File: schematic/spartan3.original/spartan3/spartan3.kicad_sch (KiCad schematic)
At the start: 245 parts, among them U1_clk_select_0 SPFT_Sliding_Switch-dynacore, U2 XC3S250E-4TQG144C

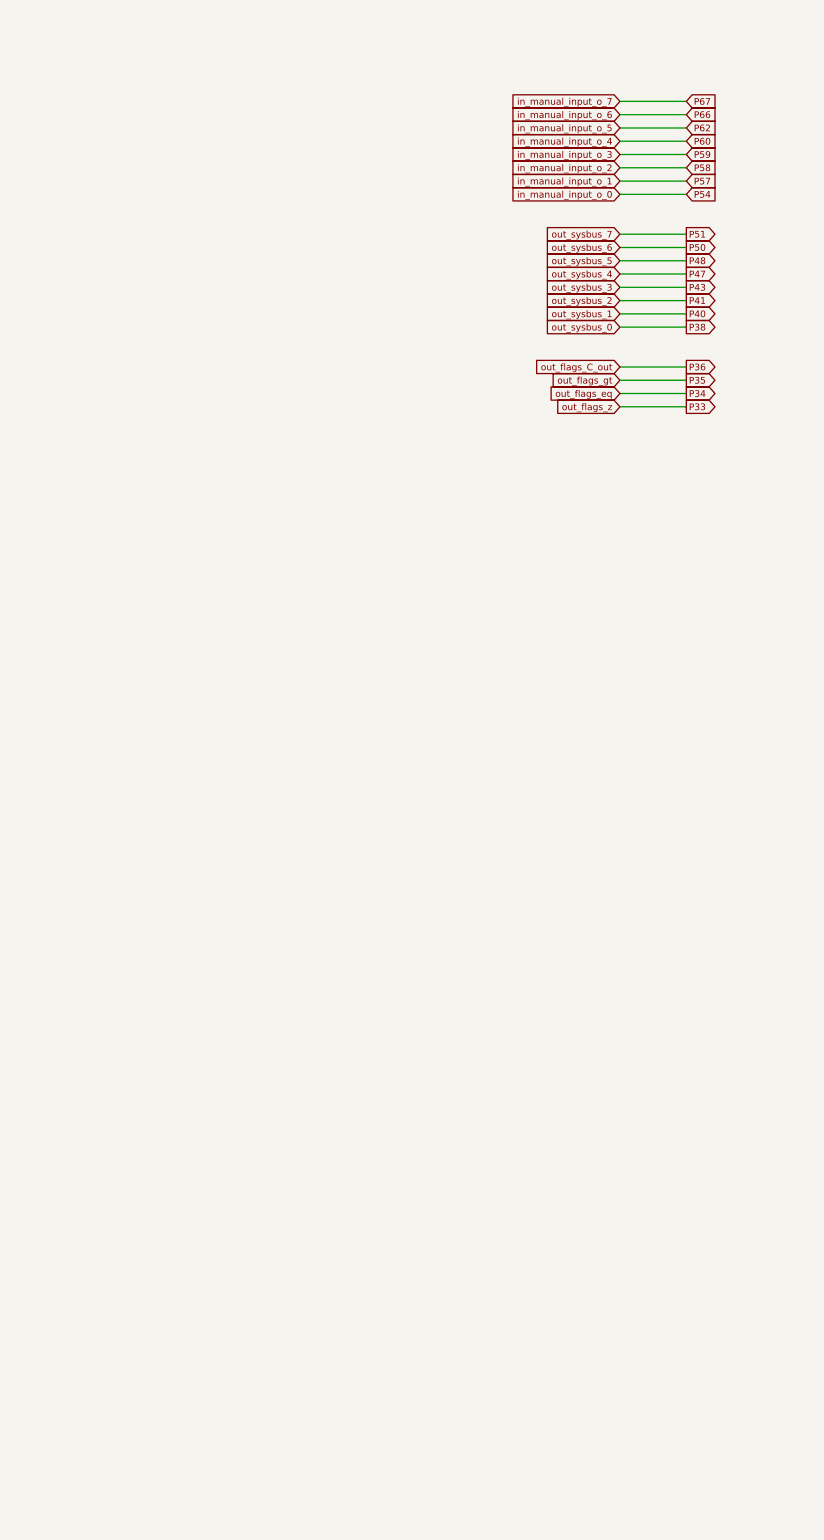
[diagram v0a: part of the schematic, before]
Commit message: Schematics :: updated. PCB layout :: updated
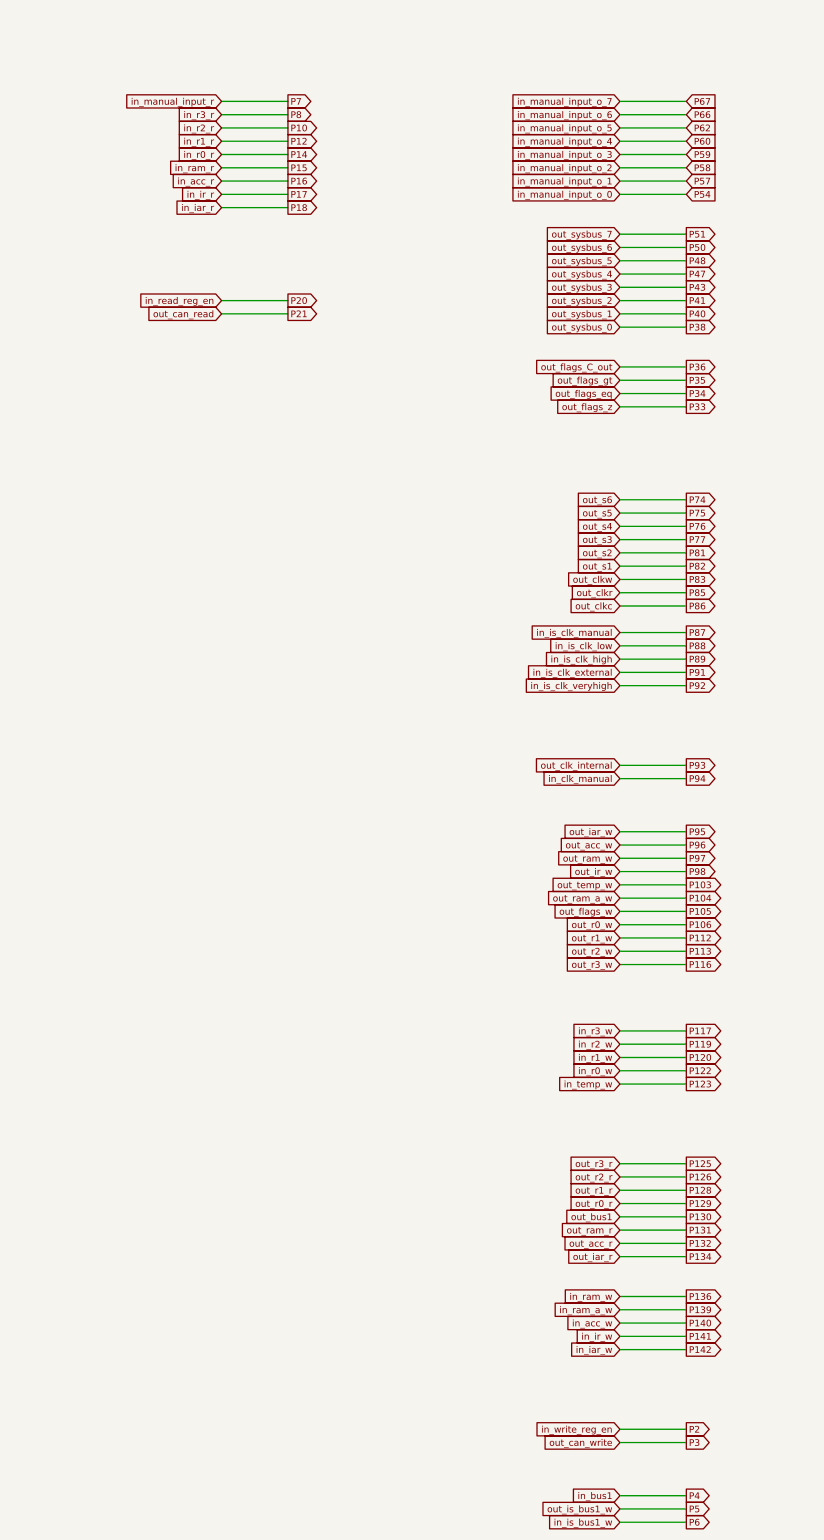
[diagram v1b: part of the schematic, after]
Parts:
- J_pwr_0: footprint Connector_USB:USB_A_Molex_67643_Horizontal -> Connector_USB:USB_A_Molex_105057_Vertical
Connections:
- net in_acc_r is gone; now on net P16: D_in_acc_r_0.1 (K), R_in_acc_r_0.1, SW_read_register_0.7
- net in_acc_w is gone; now on net P140: D_in_acc_w_0.1 (K), R_in_acc_w_0.1, SW_in_acc_w_0.5 (B)
- net in_bus1 is gone; now on net P4: D_in_bus1_one_0.1 (K), D_in_bus1_ps_0.2 (A), R_in_bus1_0.1, SW_in_bus1_0.2 (B)
- net in_clk_manual is gone; now on net P94: D_in_clk_manual_0.1 (K), R_in_clk_manual_0.1, SW_in_clk_manual_0.1
- net in_iar_r is gone; now on net P18: D_in_iar_r_0.1 (K), R_in_iar_r_0.1, SW_read_register_0.5
- net in_iar_w is gone; now on net P142: D_in_iar_w_0.1 (K), R_in_iar_w_0.1, SW_in_iar_w_0.5 (B)
- net in_ir_r is gone; now on net P17: D_in_ir_r_0.1 (K), R_in_ir_r_0.1, SW_read_register_0.6
- net in_ir_w is gone; now on net P141: D_in_ir_w_0.1 (K), R_in_ir_w_0.1, SW_in_ir_w_0.5 (B)
- net in_is_bus1_w is gone; now on net P6: D_in_is_bus1_w_0.1 (K), R_in_is_bus1_w_0.1, SW_in_is_bus1_w_0.2 (B)
- net in_is_clk_external is gone; now on net P91: D_in_is_clk_external_0.1 (K), R_in_is_clk_external_0.1, U1_clk_select_0.3 (P2)
- net in_is_clk_high is gone; now on net P89: D_in_is_clk_high_0.1 (K), R_in_is_clk_high_0.1, U1_clk_select_0.4 (P3)
- net in_is_clk_low is gone; now on net P88: D_in_is_clk_low_0.1 (K), R_in_is_clk_low_0.1, U1_clk_select_0.5 (P4)
- net in_is_clk_manual is gone; now on net P87: D_in_is_clk_manual_0.1 (K), R_in_is_clk_manual_0.1, U1_clk_select_0.6 (P5)
- net in_is_clk_veryhigh is gone; now on net P92: D_in_is_clk_veryhigh_0.1 (K), R_in_is_clk_veryhigh_0.1, U1_clk_select_0.2 (P1)
- net in_manual_input_r is gone; now on net P7: D_in_manual_input_r_0.1 (K), R_in_manual_input_r_0.1, SW_read_register_0.1
- net in_r0_r is gone; now on net P14: D_in_r0_r_0.1 (K), R_in_r0_r_0.1, SW_read_register_0.9
- net in_r0_w is gone; now on net P122: D_in_r0_w_0.1 (K), R_in_r0_w_0.1, SW_in_r0_w_0.5 (B)
- net in_r1_r is gone; now on net P12: D_in_r1_r_0.1 (K), R_in_r1_r_0.1, SW_read_register_0.10
- net in_r1_w is gone; now on net P120: D_in_r1_w_0.1 (K), R_in_r1_w_0.1, SW_in_r1_w_0.5 (B)
- net in_r2_r is gone; now on net P10: D_in_r2_r_0.1 (K), R_in_r2_r_0.1, SW_read_register_0.11
- net in_r2_w is gone; now on net P119: D_in_r2_w_0.1 (K), R_in_r2_w_0.1, SW_in_r2_w_0.5 (B)
- net in_r3_r is gone; now on net P8: D_in_r3_r_0.1 (K), R_in_r3_r_0.1, SW_read_register_0.12
- net in_r3_w is gone; now on net P117: D_in_r3_w_0.1 (K), R_in_r3_w_0.1, SW_in_r3_w_0.5 (B)
- net in_ram_a_w is gone; now on net P139: D_in_ram_a_w_0.1 (K), R_in_ram_a_w_0.1, SW_in_ram_a_w_0.5 (B)
- net in_ram_r is gone; now on net P15: D_in_ram_r_0.1 (K), R_in_ram_r_0.1, SW_read_register_0.8
- net in_ram_w is gone; now on net P136: D_in_ram_w_0.1 (K), R_in_ram_w_0.1, SW_in_ram_w_0.5 (B)
- net in_read_reg_en is gone; now on net P20: D_in_read_reg_en_0.1 (K), R_in_read_reg_en_0.1, SW_in_read_reg_en_0.2 (B)
- net in_temp_w is gone; now on net P123: D_in_temp_w_0.1 (K), R_in_temp_w_0.1, SW_in_temp_w_0.5 (B)
- net in_write_reg_en is gone; now on net P2: D_in_write_reg_en_0.1 (K), R_in_write_reg_en_0.1, SW_in_write_reg_en_0.2 (B)
- net out_acc_r is gone; now on net P132: D_out_acc_r_0.2 (A)
- net out_acc_w is gone; now on net P96: D_out_acc_w_0.2 (A)
- net out_bus1 is gone; now on net P130: D_out_bus1_0.2 (A)
- net out_can_read is gone; now on net P21: D_out_can_read_0.2 (A)
- net out_can_write is gone; now on net P3: D_out_can_write_0.2 (A)
- net out_clk_internal is gone; now on net P93: D_out_clk_internal_0.2 (A)
- net out_clkc is gone; now on net P86: D_out_clkc_0.2 (A)
- net out_clkr is gone; now on net P85: D_out_clkr_0.2 (A)
- net out_clkw is gone; now on net P83: D_out_clkw_0.2 (A)
- net out_flags_w is gone; now on net P105: D_out_flags_w_0.2 (A)
- net out_iar_r is gone; now on net P134: D_out_iar_r_0.2 (A)
- net out_iar_w is gone; now on net P95: D_out_iar_w_0.2 (A)
- net out_ir_w is gone; now on net P98: D_out_ir_w_0.2 (A)
- net out_is_bus1_w is gone; now on net P5: D_out_is_bus1_w_0.2 (A)
- net out_r0_r is gone; now on net P129: D_out_r0_r_0.2 (A)
- net out_r0_w is gone; now on net P106: D_out_r0_w_0.2 (A)
- net out_r1_r is gone; now on net P128: D_out_r1_r_0.2 (A)
- net out_r1_w is gone; now on net P112: D_out_r1_w_0.2 (A)
- net out_r2_r is gone; now on net P126: D_out_r2_r_0.2 (A)
- net out_r2_w is gone; now on net P113: D_out_r2_w_0.2 (A)
- net out_r3_r is gone; now on net P125: D_out_r3_r_0.2 (A)
- net out_r3_w is gone; now on net P116: D_out_r3_w_0.2 (A)
- net out_ram_a_w is gone; now on net P104: D_out_ram_a_w_0.2 (A)
- net out_ram_r is gone; now on net P131: D_out_ram_r_0.2 (A)
- net out_ram_w is gone; now on net P97: D_out_ram_w_0.2 (A)
- net out_s1 is gone; now on net P82: D_out_s1_0.2 (A)
- net out_s2 is gone; now on net P81: D_out_s2_0.2 (A)
- net out_s3 is gone; now on net P77: D_out_s3_0.2 (A)
- net out_s4 is gone; now on net P76: D_out_s4_0.2 (A)
- net out_s5 is gone; now on net P75: D_out_s5_0.2 (A)
- net out_s6 is gone; now on net P74: D_out_s6_0.2 (A)
- net out_temp_w is gone; now on net P103: D_out_temp_w_0.2 (A)
